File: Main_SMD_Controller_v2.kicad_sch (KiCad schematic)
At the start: 50 parts, among them J1 Vsens, J2 VsensJMP, J3 Vin+, J4 Drain, J7 Gate, J8 Source, J9 Vin_-, P1 Eoshi-chan_Silk, P2 Eoshi-chan_Silk, P3 Serial_QR, U10 TC74HC4066AP, U2 LT1167CN8, U3 TC74HC4066AP, U4 ADA4510-2ARZ, U6 ADA4522-1ARZ, U7 OP07, U9 AD633ANZ

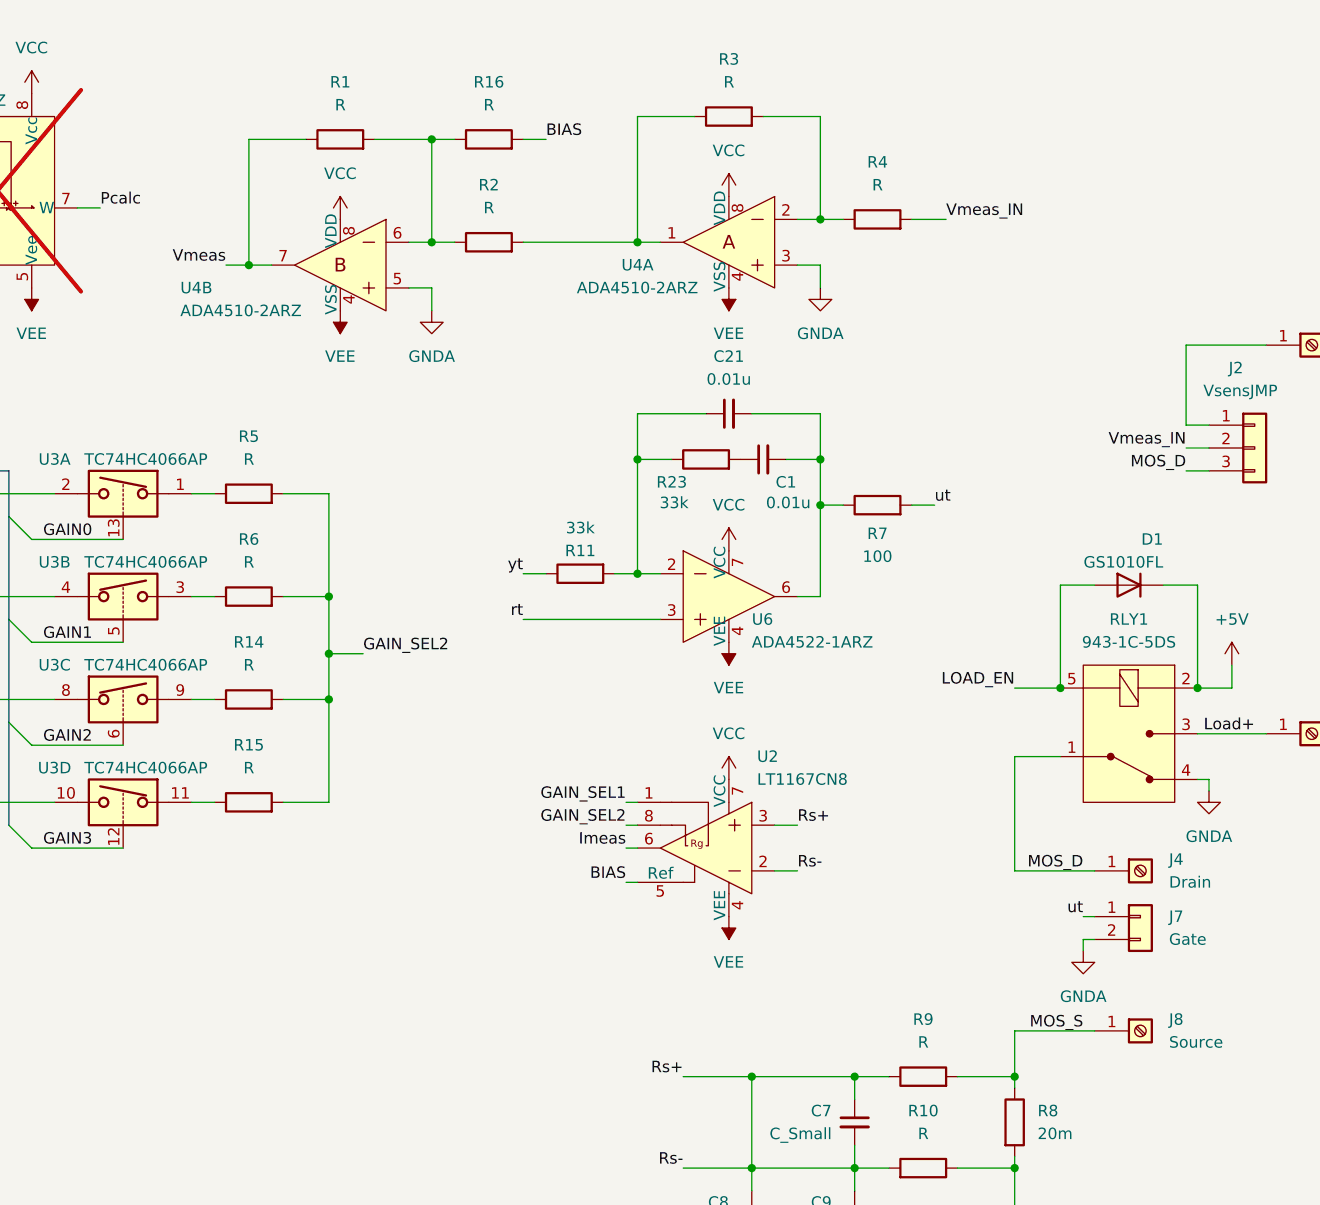
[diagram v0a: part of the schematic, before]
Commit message: 電圧
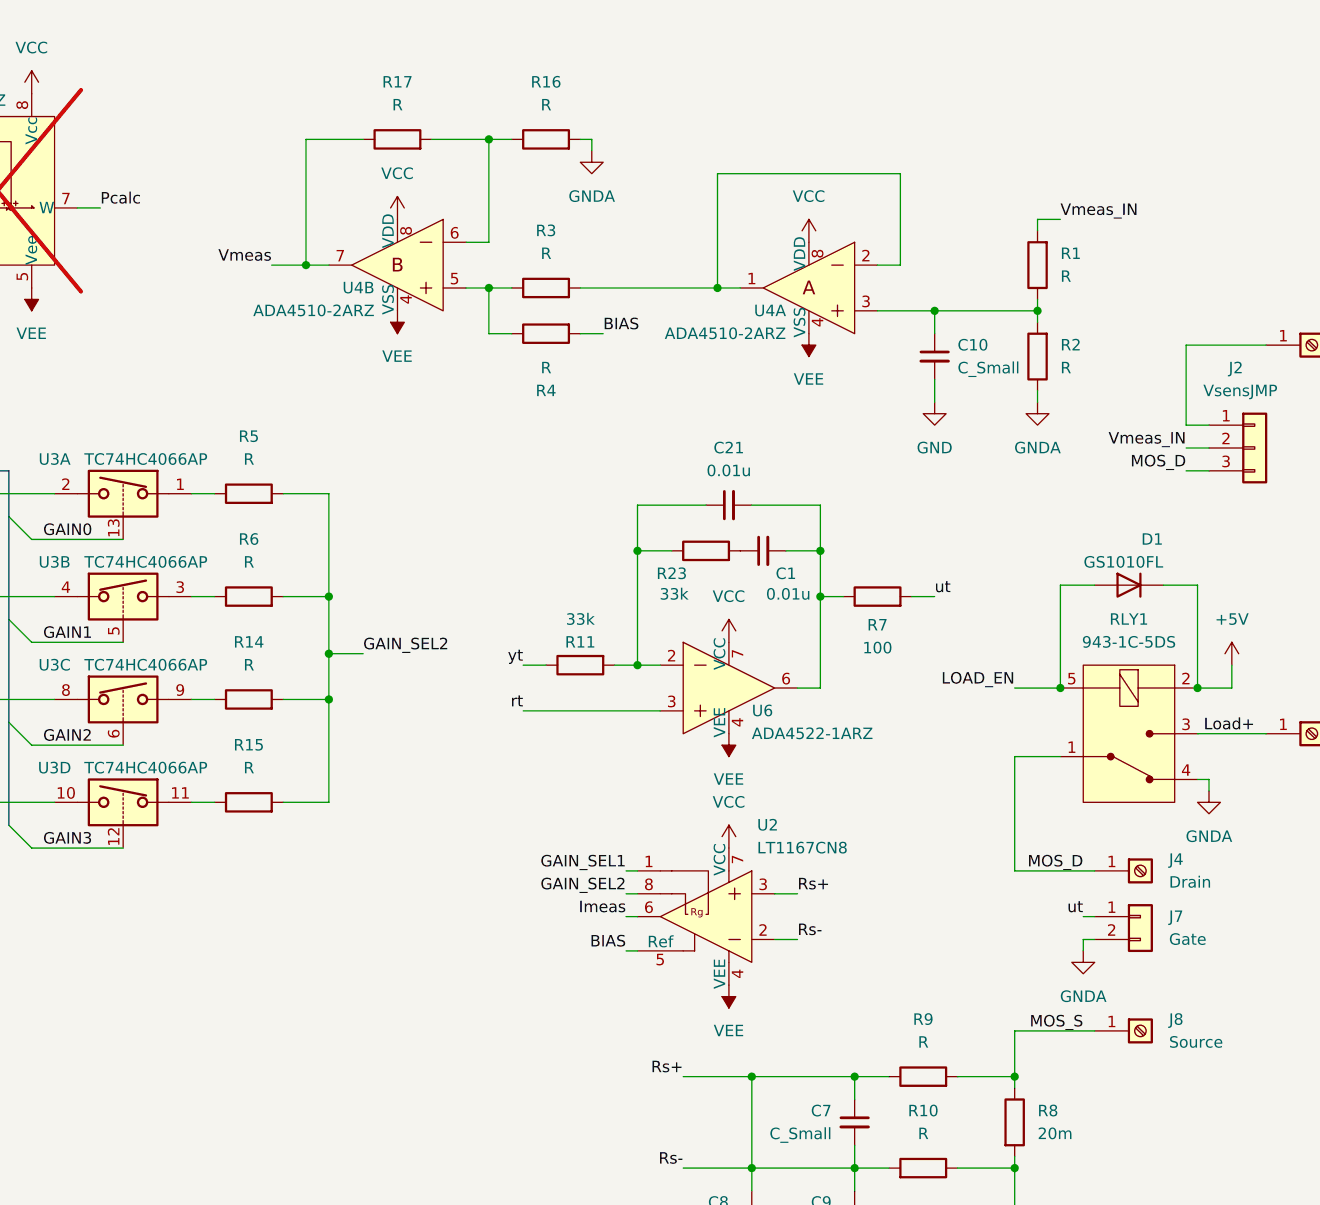
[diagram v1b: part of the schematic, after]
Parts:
- added C10: C_Small, symbol Device:C_Small
- added R17: R, symbol Device:R
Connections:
- net BIAS: now also R4.2; no longer R16.2
- net GND: now also R16.2, R2.1, C10.2; no longer U4.3, U4.5
- net Vmeas: now also R17.1; no longer R1.1
- net Vmeas_IN: now also R1.2; no longer R4.2
- net at R16.1, U4.6: now also R17.2; no longer R1.2, R2.1
- net at R3.2, U4.2: now also U4.1; no longer R4.1
- new net: C10.1, R1.1, R2.2, U4.3
- new net: R3.1, R4.1, U4.5
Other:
- moved on the sheet: C1, C21, R11, R23, R7, U2, U6
